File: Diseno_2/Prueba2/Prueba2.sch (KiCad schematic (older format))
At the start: 0 parts

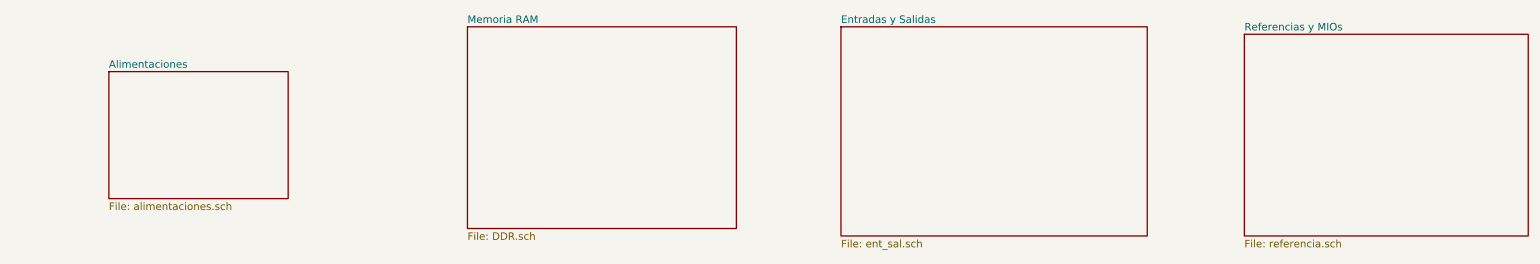
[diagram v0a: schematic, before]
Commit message: s
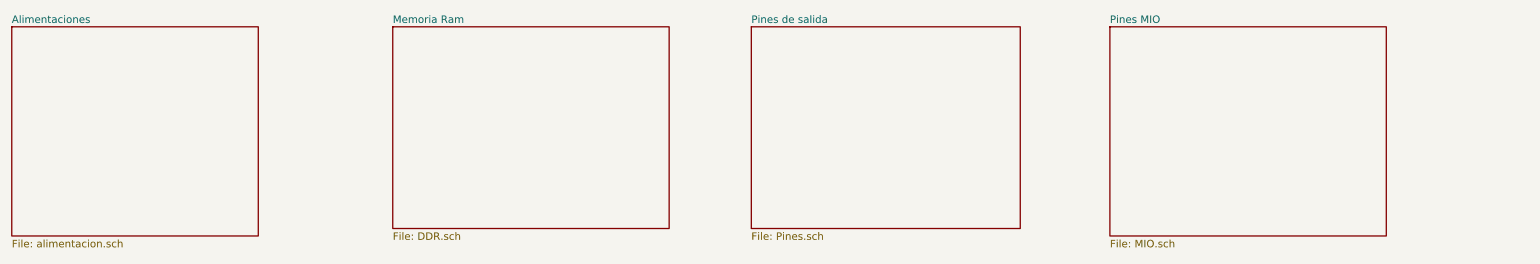
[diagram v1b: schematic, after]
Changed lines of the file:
@@
 EESchema Schematic File Version 4
-LIBS:Diseno_1-cache
 EELAYER 30 0
 EELAYER END
@@
 $EndDescr
 $Sheet
-S 3250 4450 1200 850
-U 5FFBC59B
+S 2600 4150 1650 1400
+U 5FE4D665
 F0 "Alimentaciones" 50
-F1 "alimentaciones.sch" 50
+F1 "alimentacion.sch" 50
 $EndSheet
 $Sheet
-S 5650 4150 1800 1350
-U 60C35662
-F0 "Memoria RAM" 50
+S 5150 4150 1850 1350
+U 5FE4D69B
+F0 "Memoria Ram" 50
 F1 "DDR.sch" 50
 $EndSheet
 $Sheet
-S 8150 4150 2050 1400
-U 60C66A49
-F0 "Entradas y Salidas" 50
-F1 "ent_sal.sch" 50
+S 7550 4150 1800 1350
+U 5FE4D6D0
+F0 "Pines de salida" 50
+F1 "Pines.sch" 50
 $EndSheet
 $Sheet
-S 10850 4200 1900 1350
-U 60C66A87
-F0 "Referencias y MIOs" 50
-F1 "referencia.sch" 50
+S 9950 4150 1850 1400
+U 5FE4D6FC
+F0 "Pines MIO" 50
+F1 "MIO.sch" 50
 $EndSheet
 $EndSCHEMATC
